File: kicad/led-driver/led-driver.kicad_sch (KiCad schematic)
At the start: 37 parts, among them J1 RJ45, J10 Conn_02x06_Odd_Even, J11 Conn_02x06_Odd_Even, J2 RJ45, J3 Conn_01x02_Pin, J4 Conn_02x06_Odd_Even, J5 Conn_02x06_Odd_Even, J6 Conn_02x06_Odd_Even, J7 Conn_02x06_Odd_Even, J8 Conn_02x06_Odd_Even, J9 Conn_02x06_Odd_Even, U1 LP2985-33DBVR, U2 SN65LVDS049, U3 TLC5971PWP

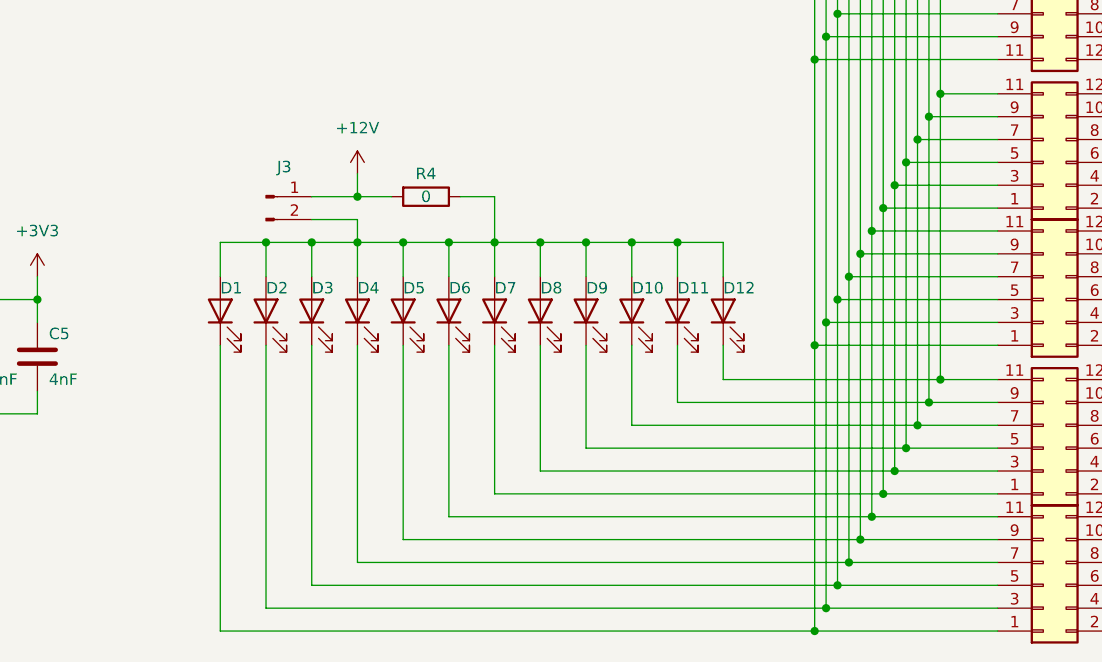
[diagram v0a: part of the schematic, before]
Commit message: Progress
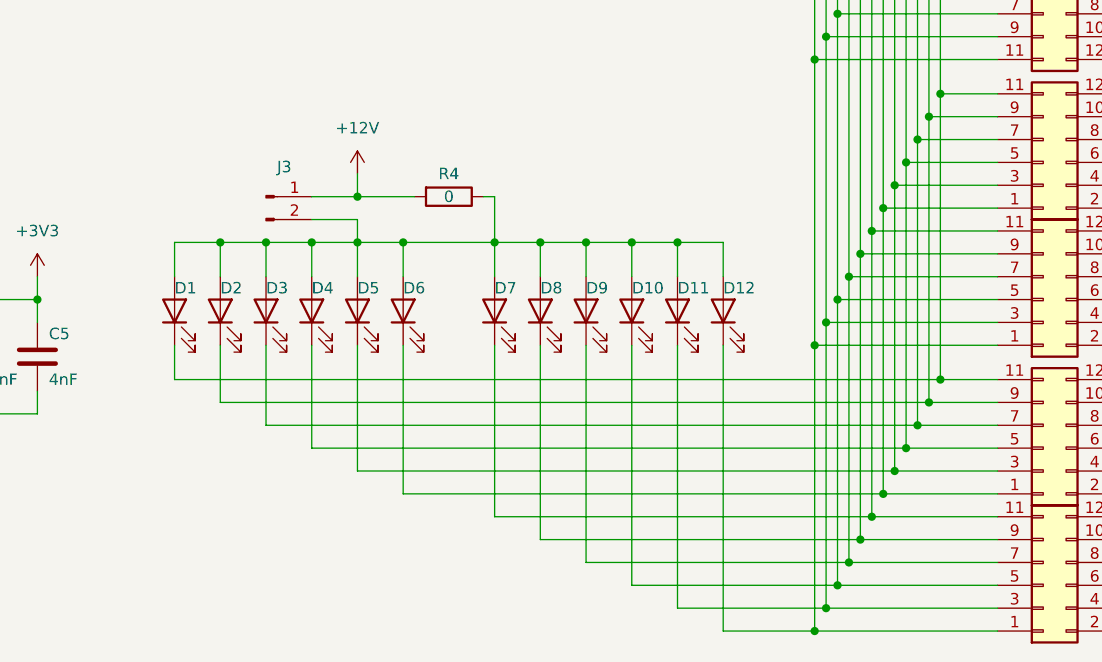
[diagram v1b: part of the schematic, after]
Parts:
- renumbered D12 to D1, D3 to D10, D2 to D11, D1 to D12, D11 to D2, D10 to D3, D9 to D4, D8 to D5, D7 to D6, D6 to D7, D5 to D8, D4 to D9
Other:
- moved on the sheet: D1, D10, D11, D12, D2, D3, D4, D5, D6, D7, D8, D9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
